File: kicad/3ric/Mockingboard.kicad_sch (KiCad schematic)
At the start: 19 parts, among them J1 Conn_01x08, J3 STX-4235-3_3-N, J4 Conn_01x08, T1_VIA1 65C22S, T2_VIA1 65C22S

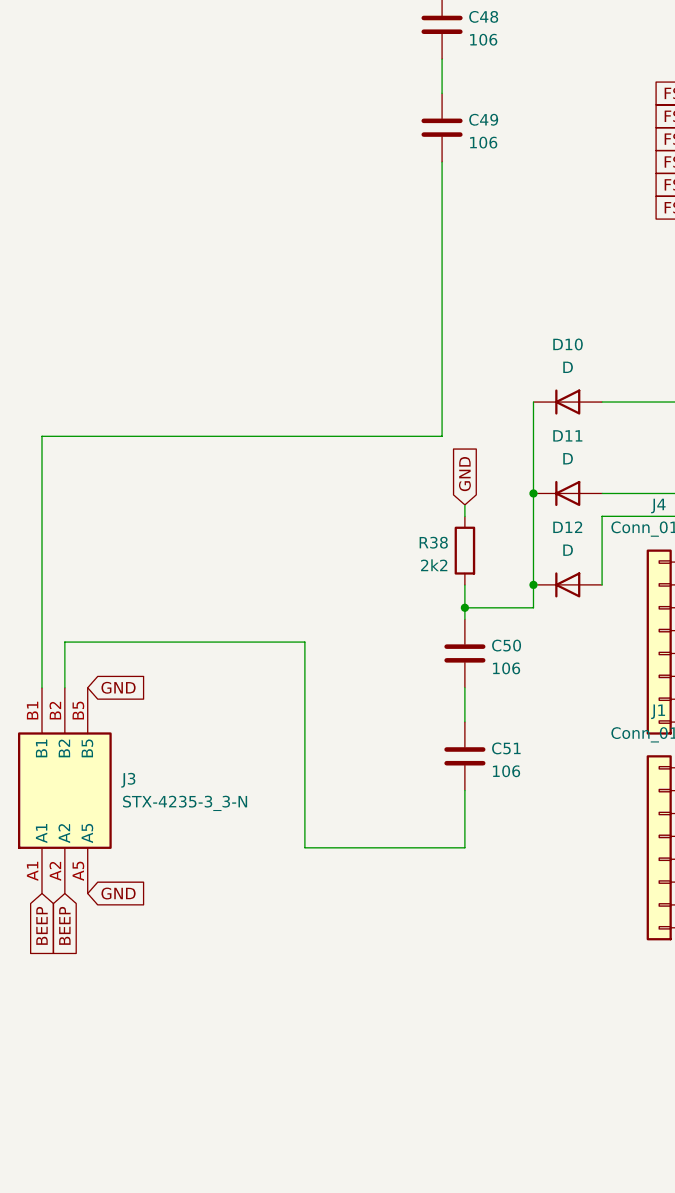
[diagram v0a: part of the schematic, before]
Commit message: pcb layout continued
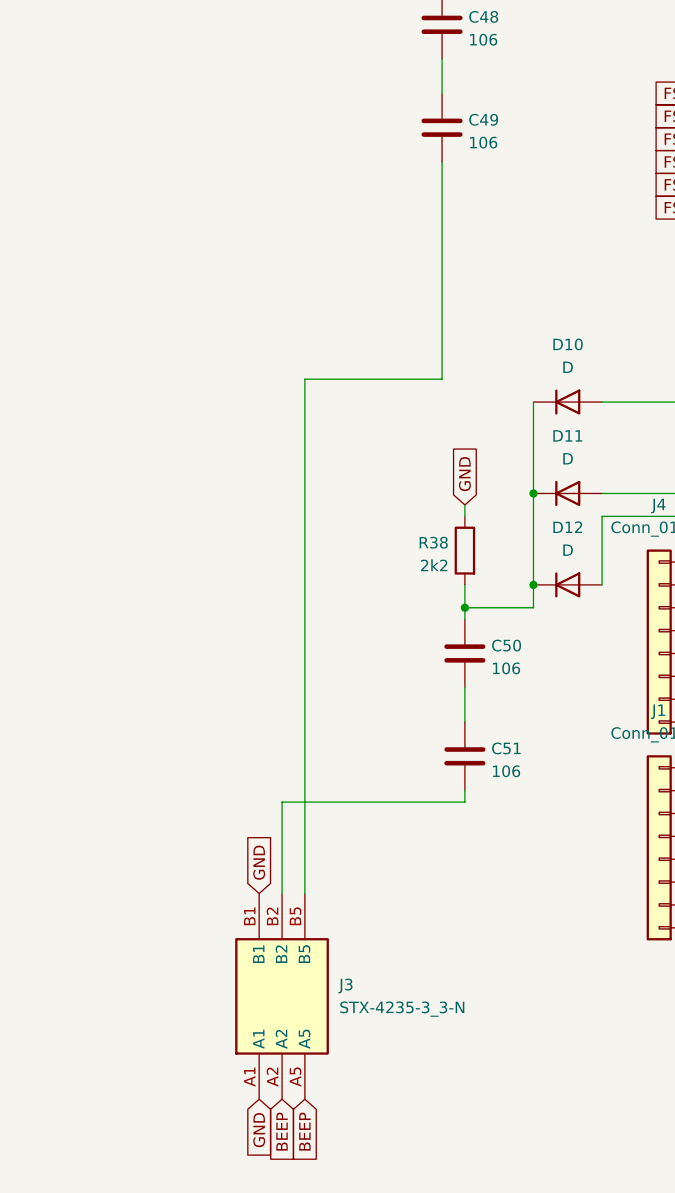
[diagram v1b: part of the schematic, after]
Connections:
- net BEEP: now also J3.A5; no longer J3.A1
- net GND: now also J3.A1, J3.B1; no longer J3.A5, J3.B5
- net at C49.2: now also J3.B5; no longer J3.B1
